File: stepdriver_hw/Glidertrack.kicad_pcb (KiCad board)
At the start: 2 copper layers, 73.2 x 38.4 mm, 51 parts, among them Q1 IRLML6302

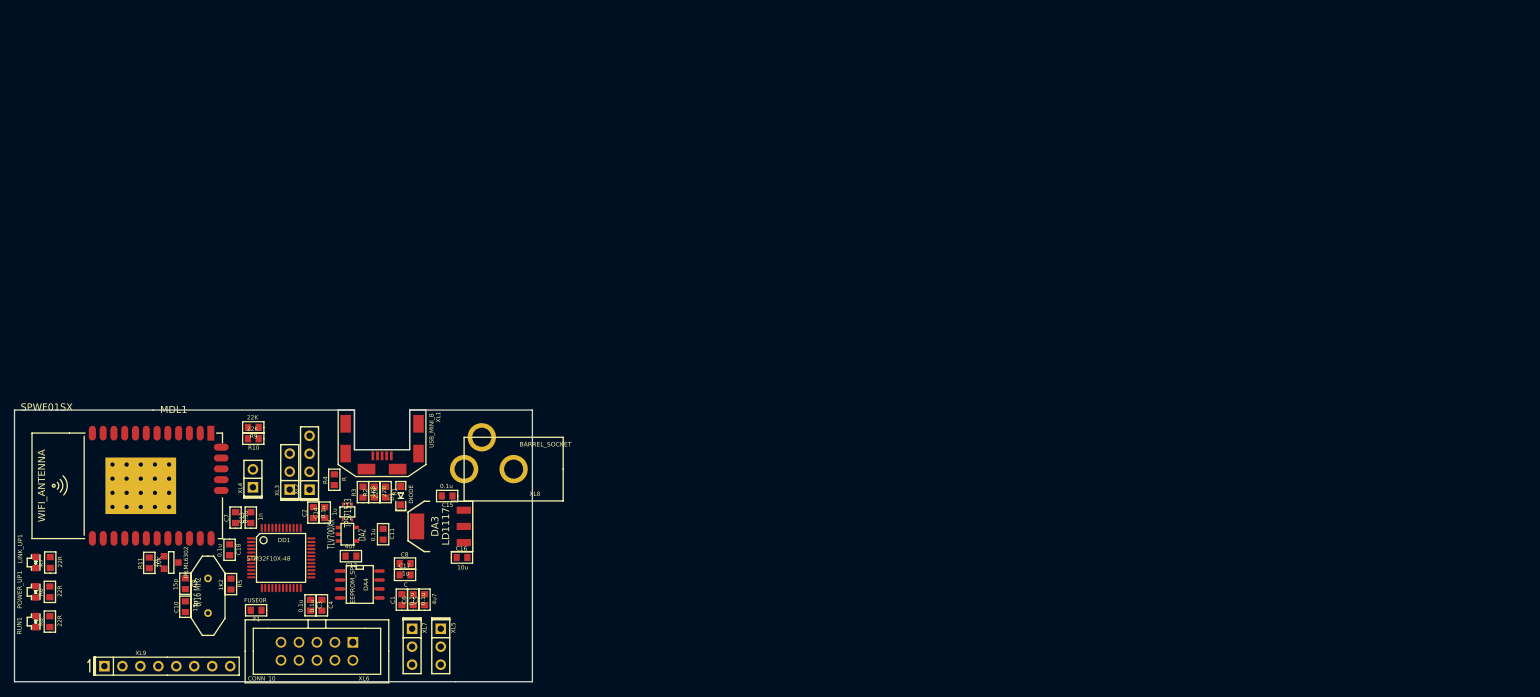
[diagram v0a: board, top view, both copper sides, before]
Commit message: HW: PCB design proceed.
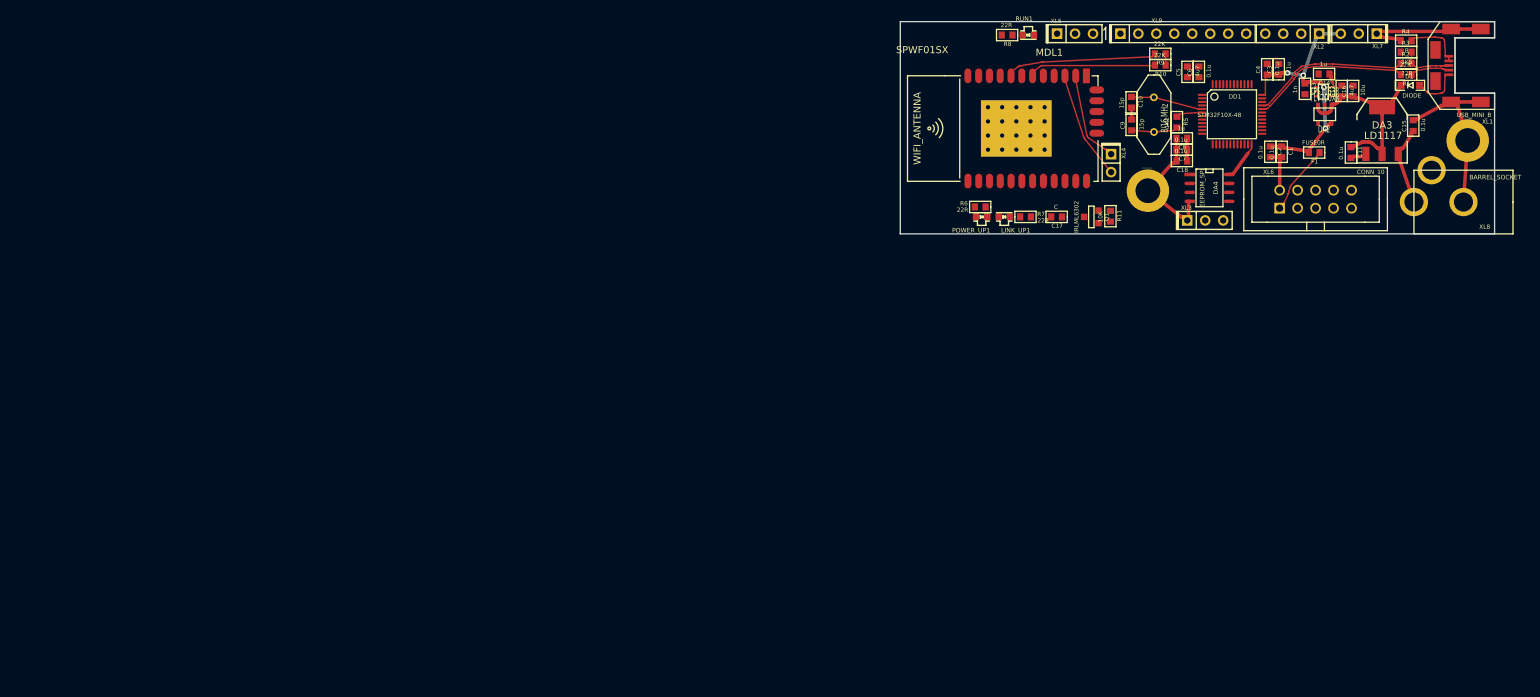
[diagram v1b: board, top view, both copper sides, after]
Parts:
- added HOLE1: HOLE_METALLED, Hole3_5_out6mm, F.Cu at (319.2, 93.8)
- added HOLE2: HOLE_METALLED, Hole3_5_out6mm, F.Cu at (274.0, 100.9)
- moved XL9 169.2 mm to (279.0, 78.7)
- moved R4 163.7 mm to (310.5, 79.7), turned to 0 degrees
- moved RUN1 163.0 mm to (257.1, 78.9), turned to 180 degrees
- moved F1 162.9 mm to (297.5, 95.5)
- moved XL1 161.1 mm to (317.4, 83.2), turned to 180 degrees
- moved C13 160.9 mm to (296.2, 86.5), turned to 270 degrees
- moved R3 160.0 mm to (310.5, 81.3), turned to 0 degrees
- moved XL7 159.4 mm to (303.8, 78.7), turned to 180 degrees
- moved R8 158.7 mm to (254.1, 78.9), turned to 180 degrees
- moved R2 157.9 mm to (310.5, 82.9), turned to 0 degrees
- moved C3 156.4 mm to (292.5, 83.7), turned to 90 degrees
- moved R1 155.8 mm to (310.5, 84.5), turned to 180 degrees
- moved XL6 154.9 mm to (297.7, 102.1), turned to 0 degrees
- moved C12 154.7 mm to (301.4, 86.8), turned to 90 degrees
- moved C14 154.3 mm to (298.9, 84.4), turned to 180 degrees
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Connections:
- C17 pad 1: N-0000083 -> N-0000081
- DD1 pad 39: /GPIOB3 -> /WIFI_PWR
- MDL1 pad 24: N-0000083 -> N-0000081
- Q1 pad 3: N-0000083 -> N-0000081
- R10 pad 1: N-0000083 -> +3.3V
- R9 pad 1: N-0000083 -> +3.3V
- XL9 pad 8: /GPIOB3 -> +3.3V
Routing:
- net GND: track 0.00 -> 73.3 mm
- net +3.3V: track 0.00 -> 54.3 mm, vias 0 -> 4
- net +5V: track 0.00 -> 29.7 mm
- net /USB_DM: track 0.00 -> 22.5 mm
- net /USB_DP: track 0.00 -> 22.5 mm
- net /WIFI_TX: track 0.00 -> 21.4 mm
- net /WIFI_RX: track 0.00 -> 18.1 mm
- net /WIFI_RESET: track 0.00 -> 15.4 mm
- net /WIFI_BOOT: track 0.00 -> 13.0 mm
- net +12V: track 0.00 -> 11.3 mm
- net N-0000080: track 0.00 -> 10.8 mm
- net N-000003: track 0.00 -> 9.88 mm
- net N-0000069: track 0.00 -> 8.32 mm
- net N-0000077: track 0.00 -> 7.19 mm
- net N-0000082: track 0.00 -> 6.88 mm
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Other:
- board size 73.2 x 38.4 mm -> 84 x 30 mm
